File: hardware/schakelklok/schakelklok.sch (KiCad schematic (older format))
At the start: 9 parts

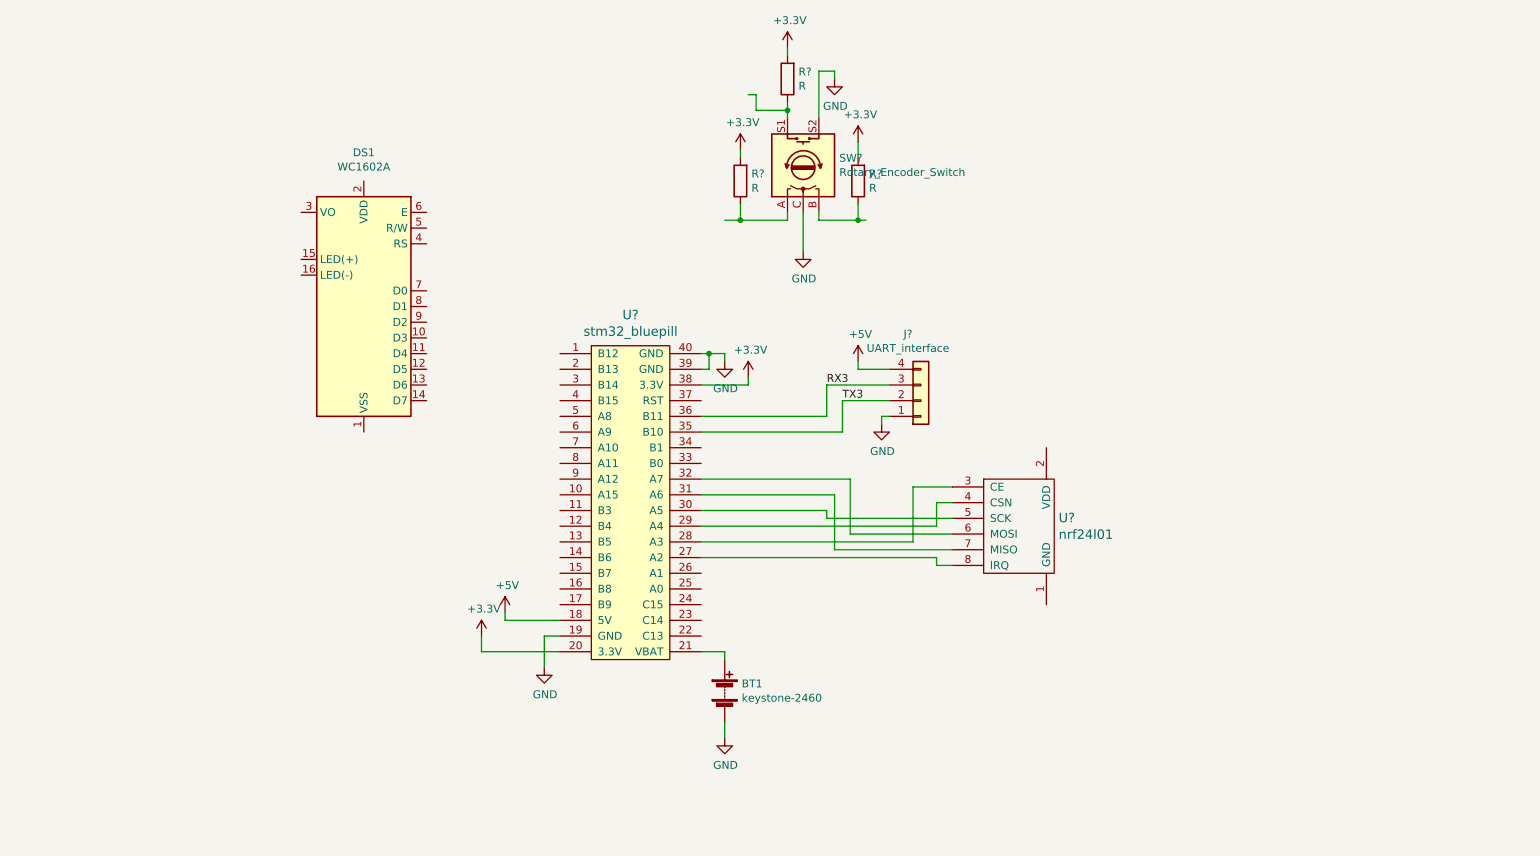
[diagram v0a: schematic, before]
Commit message: finished schematic
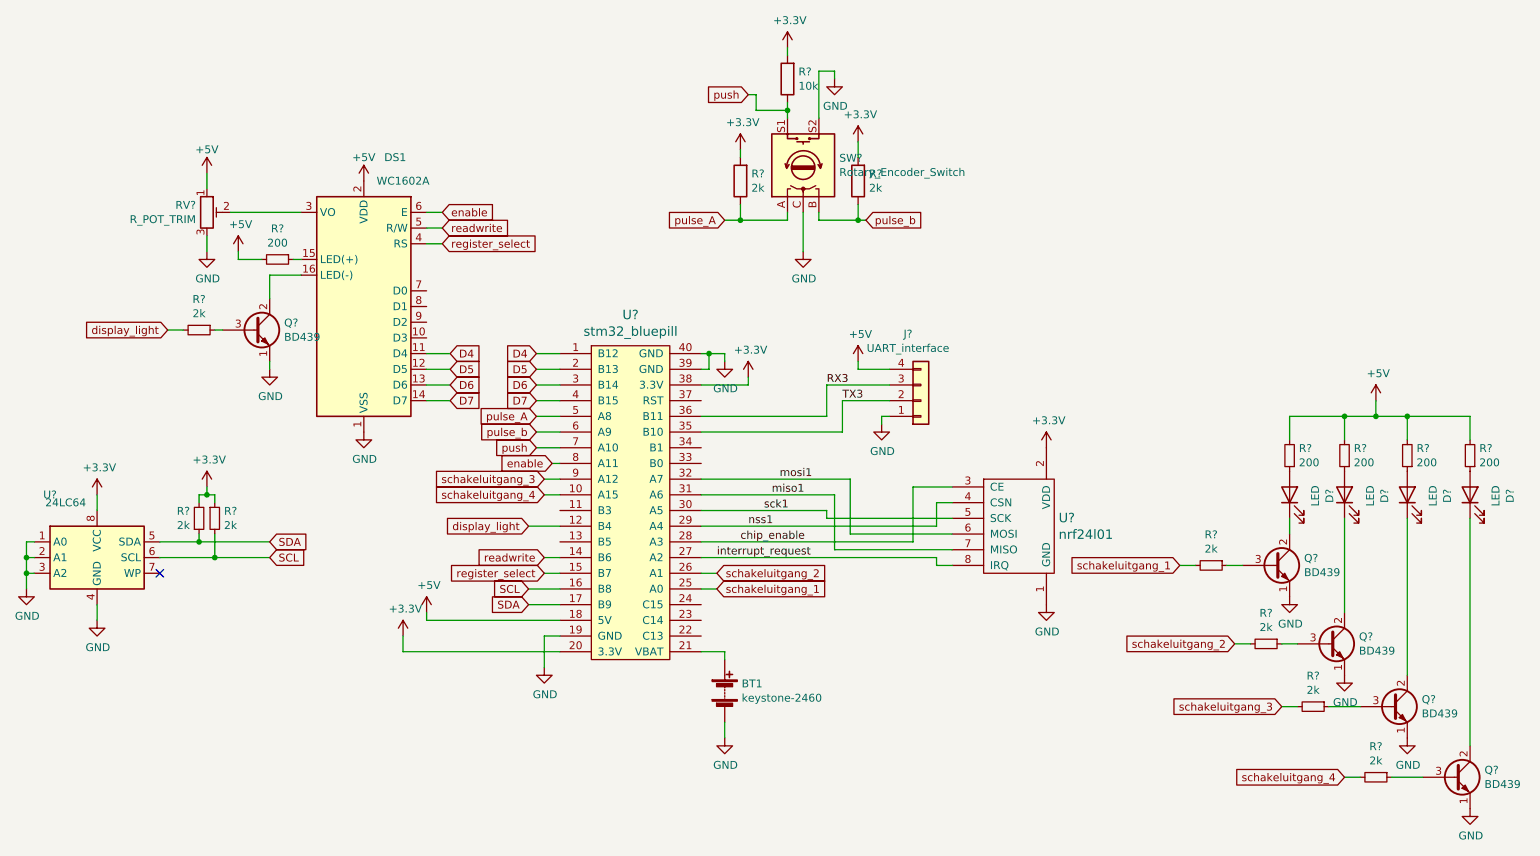
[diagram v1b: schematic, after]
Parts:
- added D? (x4): LED, symbol Device:LED
- added Q? (x5): BD439, Package_TO_SOT_THT:TO-126-3_Vertical, symbol Transistor_BJT:BD439
- added R? (x7): 2k, symbol Device:R_Small
- added R? (x5): 200, symbol Device:R_Small
- added RV?: R_POT_TRIM, symbol Device:R_POT_TRIM
- added U?: 24LC64, symbol Memory_EEPROM:24LC64
- R? (x2): value R -> 2k
- R?: value R -> 10k
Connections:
- net labels added: D4, D5, D6, D7, SCL, SDA, chip_enable, display_light, enable, interrupt_request, miso1, mosi1, nss1, pulse_A, pulse_b, push, readwrite, register_select, schakeluitgang_1, schakeluitgang_2, schakeluitgang_3, schakeluitgang_4, sck1
- wire segments 64 -> 139
- no-connect marks 0 -> 1
